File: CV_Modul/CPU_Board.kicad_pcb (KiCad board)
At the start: 4 copper layers, 65 x 100 mm, 127 parts, among them J101 Screw_Terminal_01x03, J102 Conn_02x01, J103 Conn_02x01, J104 Conn_01x08_Male, J105 Conn_02x09_Odd_Even, J106 Micro_SD_Card_Det, J107 Conn_01x06_Male, J108 Conn_02x01, J109 Conn_02x01, J110 Screw_Terminal_01x04, J111 Conn_02x01, J112 IPC 16P, SW1 SW_DIP_x04, SW101 Rotary_Encoder_Switch, SW102 SW_Push, U101 STM32H730ZB, U102 W9864G6KH, U103 TPS560430, U104 TPS560430, U105 SN65HVD230, U106 IDC Connector 18P, U107 IDC Connector 18P, Y101 48MHz

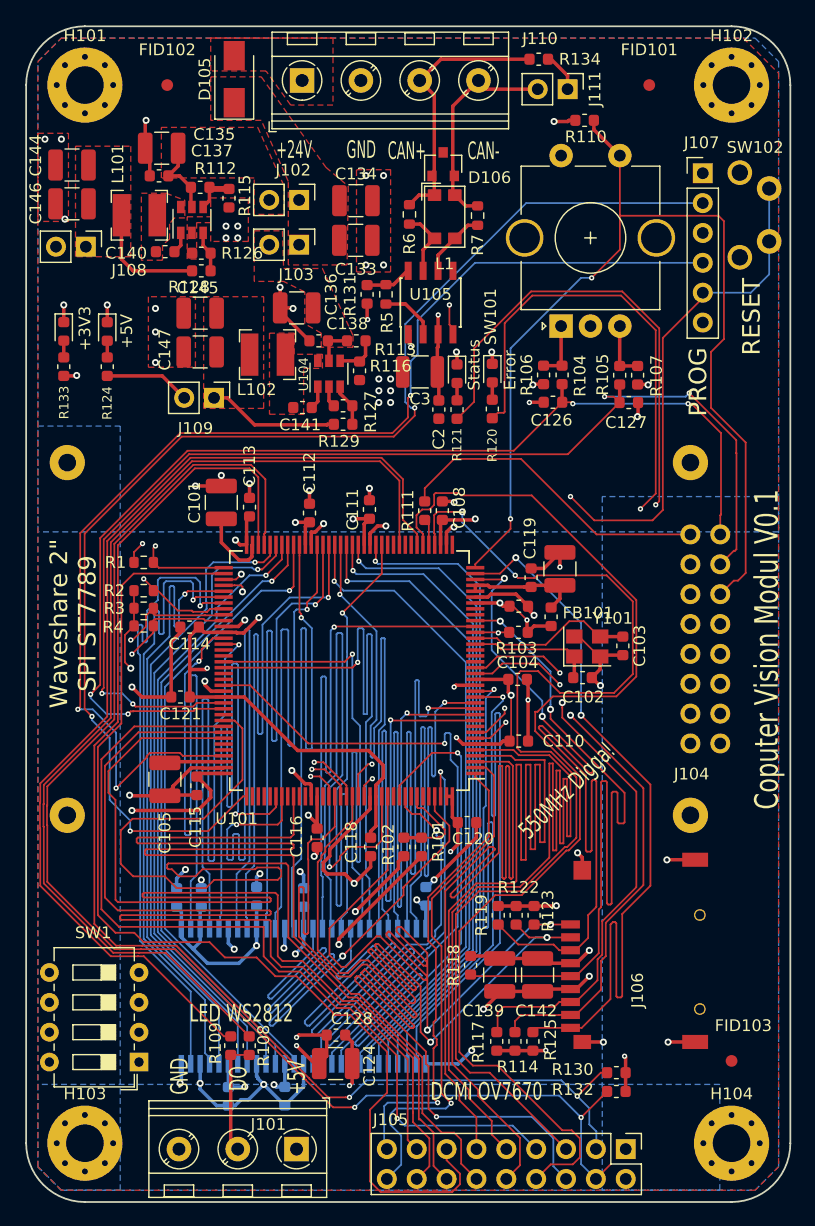
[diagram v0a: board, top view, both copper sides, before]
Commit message: Änderungen für bestellung V01 -  Bestellung abgeschickt
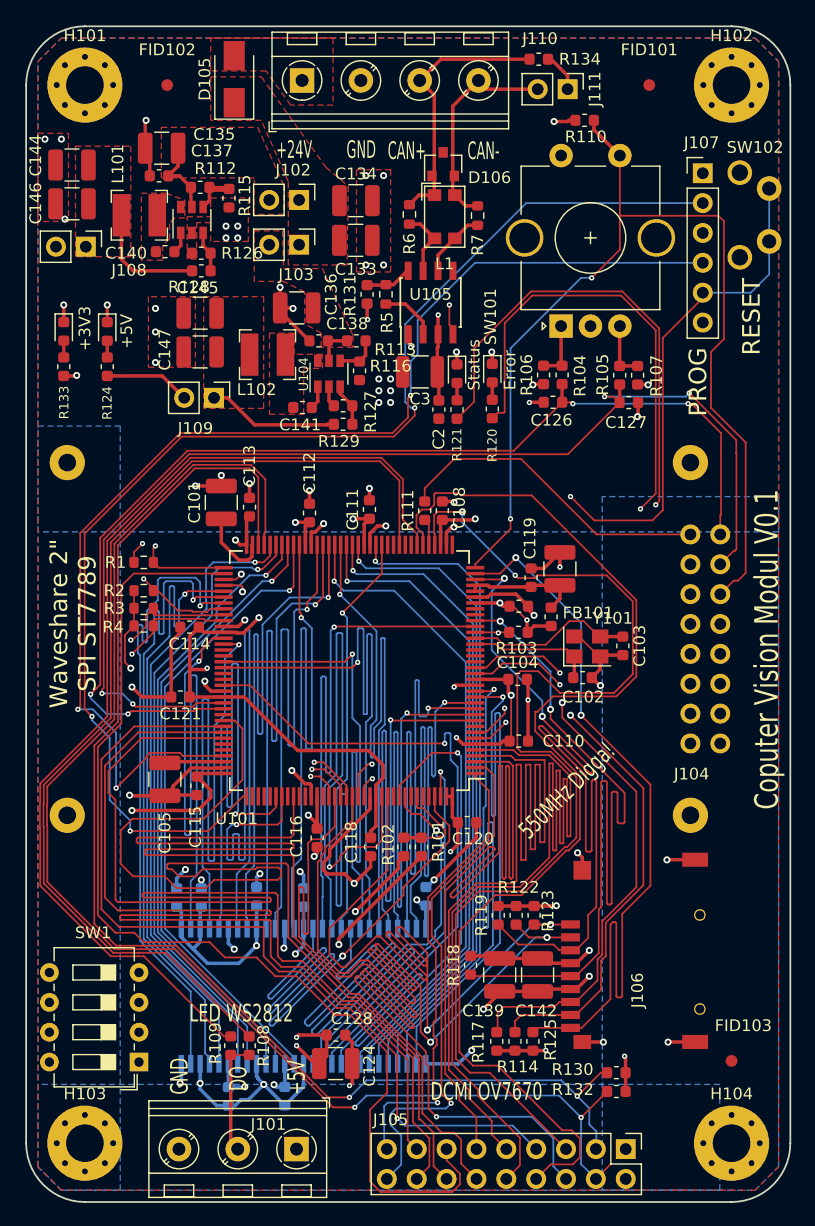
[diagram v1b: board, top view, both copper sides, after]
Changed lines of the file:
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@@
       (outputformat 1)
       (mirror false)
-      (drillshape 1)
+      (drillshape 0)
       (scaleselection 1)
-      (outputdirectory ""))
+      (outputdirectory "/home/nk/Dokumente/Pick_n_Place/02_Electric/export/CV_Modul/"))
   )
   (net 0 "")
@@
     (add_net "Net-(D105-Pad2)")
     (add_net "Net-(J101-Pad2)")
-    (add_net "Net-(J104-Pad12)")
-    (add_net "Net-(J104-Pad13)")
-    (add_net "Net-(J104-Pad14)")
-    (add_net "Net-(J104-Pad15)")
-    (add_net "Net-(J104-Pad16)")
-    (add_net "Net-(J107-Pad6)")
     (add_net "Net-(J111-Pad1)")
     (add_net "Net-(L1-Pad1)")
@@
     (add_net "Net-(R127-Pad2)")
     (add_net "Net-(R131-Pad2)")
-    (add_net "Net-(U101-Pad103)")
-    (add_net "Net-(U101-Pad104)")
-    (add_net "Net-(U101-Pad110)")
-    (add_net "Net-(U101-Pad111)")
-    (add_net "Net-(U101-Pad112)")
-    (add_net "Net-(U101-Pad113)")
-    (add_net "Net-(U101-Pad116)")
-    (add_net "Net-(U101-Pad118)")
-    (add_net "Net-(U101-Pad119)")
-    (add_net "Net-(U101-Pad122)")
-    (add_net "Net-(U101-Pad134)")
-    (add_net "Net-(U101-Pad137)")
-    (add_net "Net-(U101-Pad139)")
-    (add_net "Net-(U101-Pad140)")
-    (add_net "Net-(U101-Pad20)")
-    (add_net "Net-(U101-Pad21)")
-    (add_net "Net-(U101-Pad22)")
-    (add_net "Net-(U101-Pad28)")
-    (add_net "Net-(U101-Pad29)")
-    (add_net "Net-(U101-Pad37)")
-    (add_net "Net-(U101-Pad44)")
-    (add_net "Net-(U101-Pad45)")
-    (add_net "Net-(U101-Pad47)")
-    (add_net "Net-(U101-Pad48)")
-    (add_net "Net-(U101-Pad87)")
-    (add_net "Net-(U101-Pad88)")
-    (add_net "Net-(U101-Pad9)")
-    (add_net "Net-(U101-Pad91)")
-    (add_net "Net-(U101-Pad92)")
-    (add_net "Net-(U101-Pad98)")
-    (add_net "Net-(U102-Pad36)")
-    (add_net "Net-(U102-Pad40)")
-    (add_net "Net-(U105-Pad5)")
   )
   (net_class 50OhmS ""
@@
       (effects (font (size 1 1) (thickness 0.15)))
     )
-    (fp_text user %R (at 0 0) (layer F.Fab)
-      (effects (font (size 0.5 0.5) (thickness 0.075)))
-    )
     (fp_line (start -0.7 -0.95) (end -0.7 1.5) (layer F.Fab) (width 0.1))
     (fp_line (start -0.15 -1.52) (end 0.7 -1.52) (layer F.Fab) (width 0.1))
@@
     (fp_line (start 0.76 -1.58) (end -1.4 -1.58) (layer F.SilkS) (width 0.12))
     (fp_line (start 0.76 1.58) (end -0.7 1.58) (layer F.SilkS) (width 0.12))
+    (fp_text user %R (at 0 0) (layer F.Fab)
+      (effects (font (size 0.5 0.5) (thickness 0.075)))
+    )
     (pad 3 smd rect (at 1 0 90) (size 0.9 0.8) (layers F.Cu F.Paste F.Mask)
       (net 1 GND))
@@
       (effects (font (size 0.8 0.8) (thickness 0.12)))
     )
-    (pad 1 smd roundrect (at -1.475 0 180) (size 1.15 2.7) (layers F.Cu F.Paste F.Mask) (roundrect_rratio 0.217391)
+    (pad 1 smd roundrect (at -1.475 0 180) (size 1.15 2.7) (layers F.Cu F.Paste F.Mask) (roundrect_rratio 0.2173904347826087)
       (net 5 +3V3))
-    (pad 2 smd roundrect (at 1.475 0 180) (size 1.15 2.7) (layers F.Cu F.Paste F.Mask) (roundrect_rratio 0.217391)
+    (pad 2 smd roundrect (at 1.475 0 180) (size 1.15 2.7) (layers F.Cu F.Paste F.Mask) (roundrect_rratio 0.2173904347826087)
       (net 1 GND))
     (model ${KISYS3DMOD}/Capacitor_SMD.3dshapes/C_1210_3225Metric.wrl
@@
       (pts
         (xy 134 147) (xy 132 149) (xy 73 149) (xy 71 147) (xy 71 53)
-        (xy 73 51) (xy 131 51) (xy 134 54)
+        (xy 73 51) (xy 132 51) (xy 134 53)
       )
     )
